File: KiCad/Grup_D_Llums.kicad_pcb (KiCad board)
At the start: 2 copper layers, 122.8 x 103.7 mm, 93 parts, among them J1 DE9_Pins, J2 Screw_Terminal_01x02, J3 Screw_Terminal_01x02, J4 Conn_PIC_ICSP_ICD, J5 DE9_Pins, J6 Screw_Terminal_01x02, J7 Conn_01x10_Pin, Q1 AO3400A, Q2 AO3400A, Q3 AO3400A, Q4 AO3400A, Q5 AO3400A, Q6 AO3400A, Q7 AO3400A, Q8 AO3400A, SW1 SW_Push, SW2 SW_SPDT, SW3 SW_SPDT, SW4 SW_SPDT, SW5 SW_SPDT, SW6 SW_SPDT, SW7 SW_SPST, U1 PIC32MX250F128D-IPT, U2 LM2596S-5, U3 L298N, U6 SN65HVD232, U7 LM1117DT-3.3, U9 RPR-0521RS, Y2 Crystal

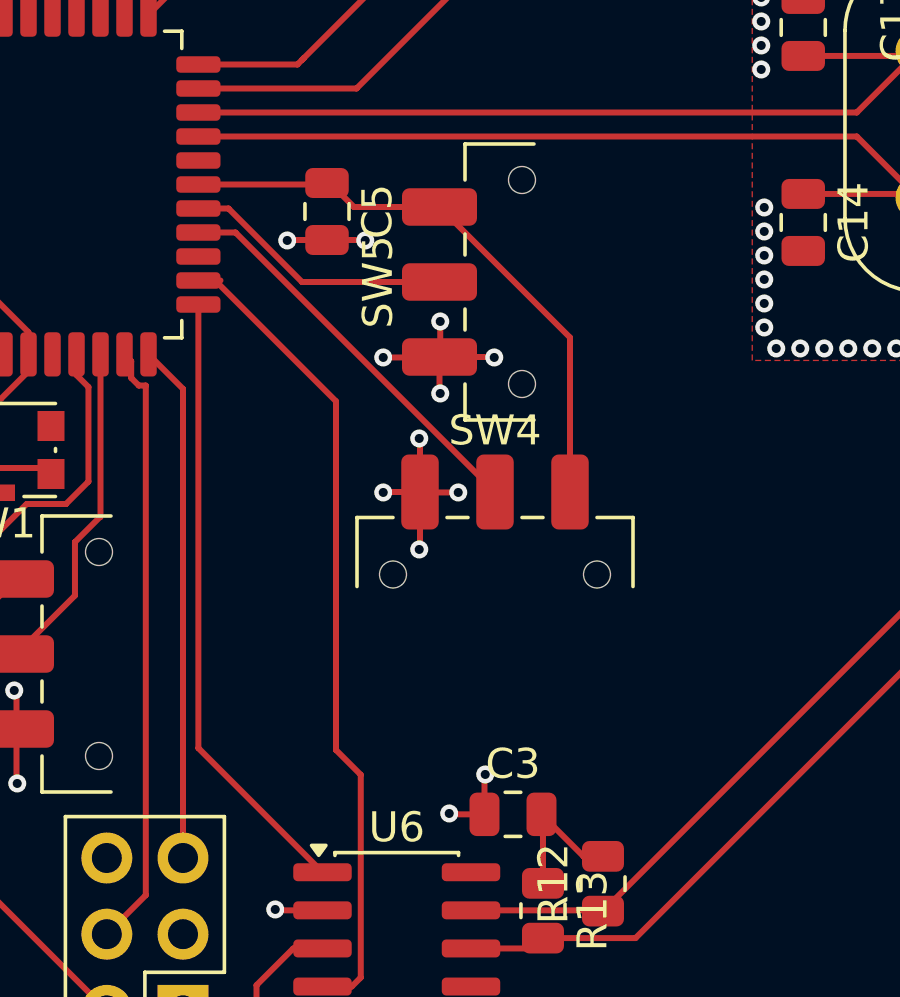
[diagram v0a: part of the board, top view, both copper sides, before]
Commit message: hotfix
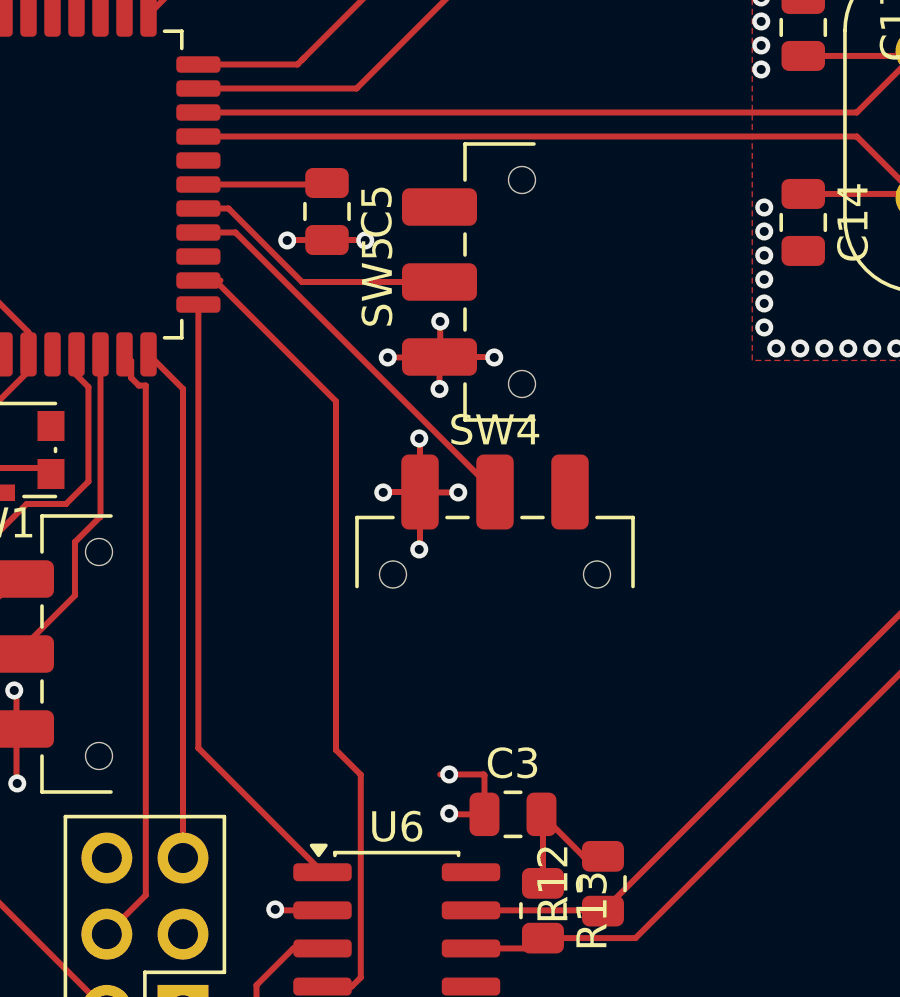
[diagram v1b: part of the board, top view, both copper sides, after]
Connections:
- net Net-(D1-K) renamed OUTLM
- net Net-(D3-K) renamed VIN
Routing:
- net VCC: track 140.7 -> 125.4 mm
- net GND: track 144.5 -> 145.7 mm
